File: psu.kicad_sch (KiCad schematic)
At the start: 12 parts, among them J1 Power in, U2 3.3v REG

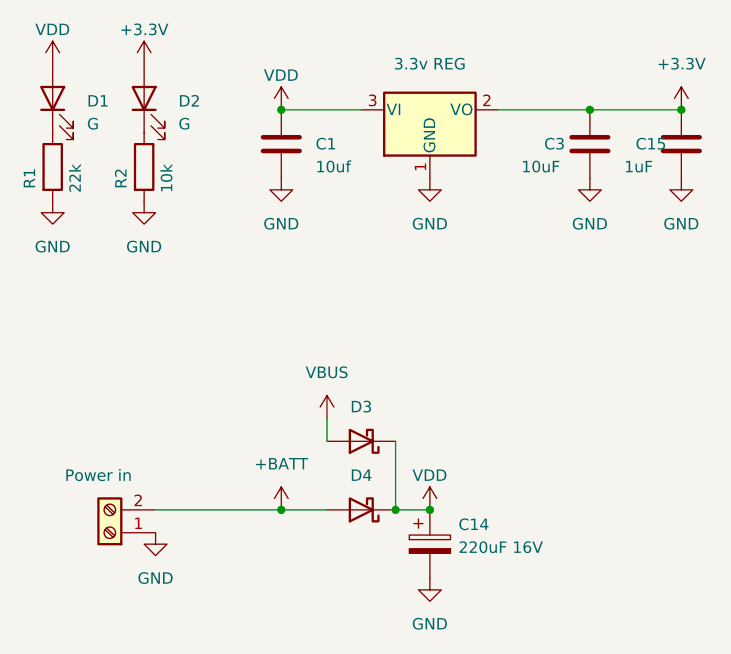
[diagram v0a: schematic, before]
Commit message: Rev 27052023
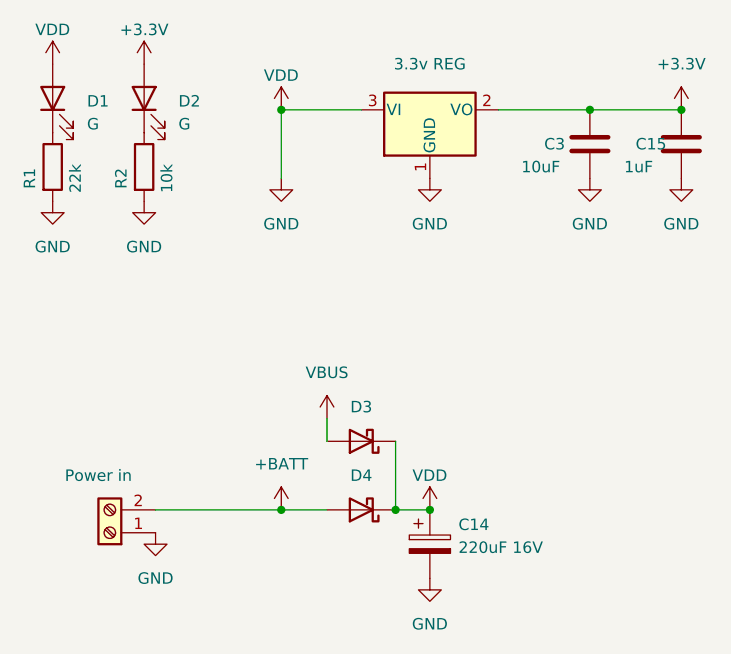
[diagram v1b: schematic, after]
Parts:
- removed C1: 10uf, Capacitor_SMD:C_0402_1005Metric_Pad0.74x0.62mm_HandSolder, symbol Device:C
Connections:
- net VDD is gone; now on net GND: C14.1, D1.2 (A), D3.1 (K), D4.1 (K), U2.3 (VI)
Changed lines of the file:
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@@
   (junction (at 50.8 83.82) (diameter 0) (color 0 0 0 0)
+  )
+  (wire (pts (xy 50.8 39.37) (xy 50.8 46.99))
+    (stroke (width 0) (type default) (color 0 0 0 0))
   )
   (wire (pts (xy 50.8 39.37) (xy 59.69 39.37))
@@
       (effects (font (size 1.27 1.27)) hide)
     )
-    (pin "1")
-    (pin "2")
-  )
-  (symbol (lib_id "Device:C") (at 50.8 43.18 0) (unit 1)
-    (in_bom yes) (on_board yes)
-    (property "Reference" "C1" (id 0) (at 54.61 43.18 0)
-      (effects (font (size 1.27 1.27)) (justify left))
-    )
-    (property "Value" "10uf" (id 1) (at 54.61 45.72 0)
-      (effects (font (size 1.27 1.27)) (justify left))
-    )
-    (property "Footprint" "Capacitor_SMD:C_0402_1005Metric_Pad0.74x0.62mm_HandSolder" (id 2) (at 51.7652 46.99 0)
-      (effects (font (size 1.27 1.27)) hide)
-    )
-    (property "Datasheet" "~" (id 3) (at 50.8 43.18 0)
-      (effects (font (size 1.27 1.27)) hide)
-    )
